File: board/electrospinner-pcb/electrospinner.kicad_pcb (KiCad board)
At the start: 2 copper layers, 50.8 x 38.1 mm, 35 parts, among them SW1 ResetBTN, U1 FT230XS, U2 TPS62147, U3 TPS62147, U4 A4988SETTR-T, U5 MSP430G2553IPW20

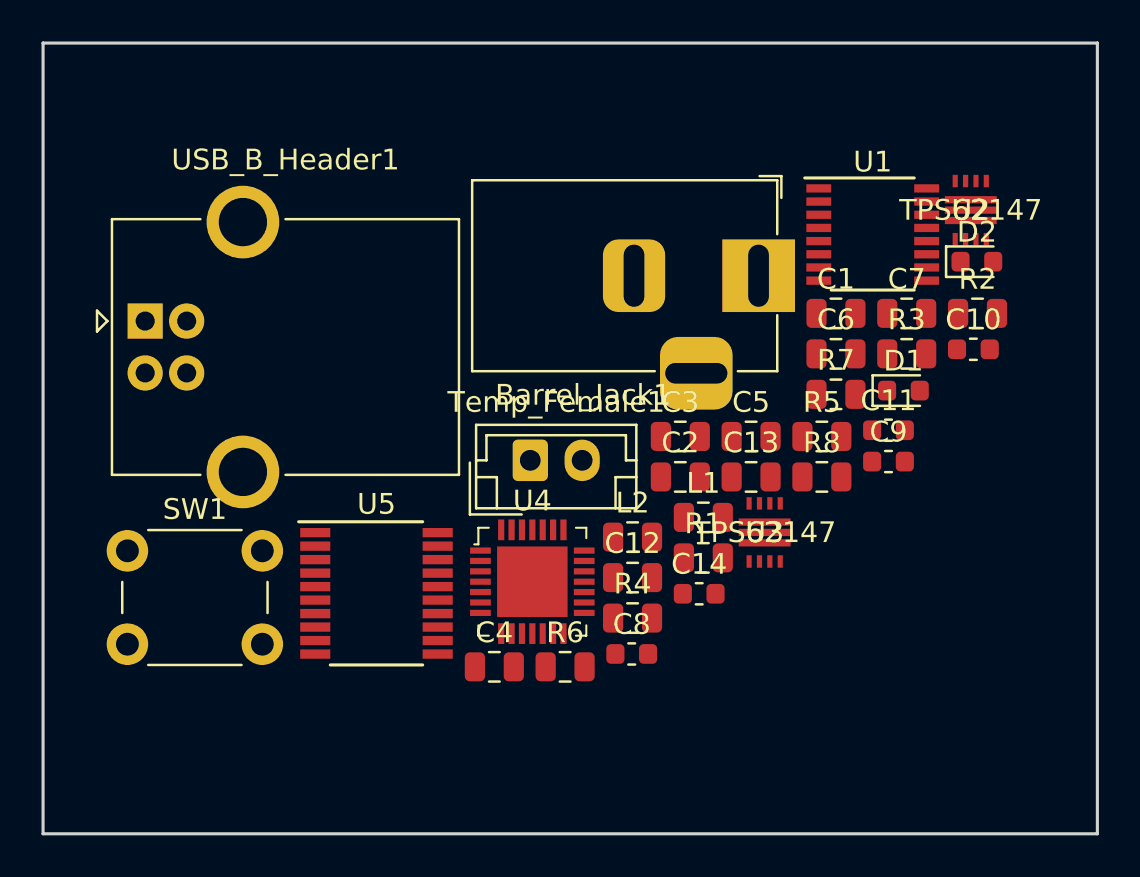
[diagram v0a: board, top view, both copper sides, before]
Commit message: Updates BOM and footprints, adds spreadsheet
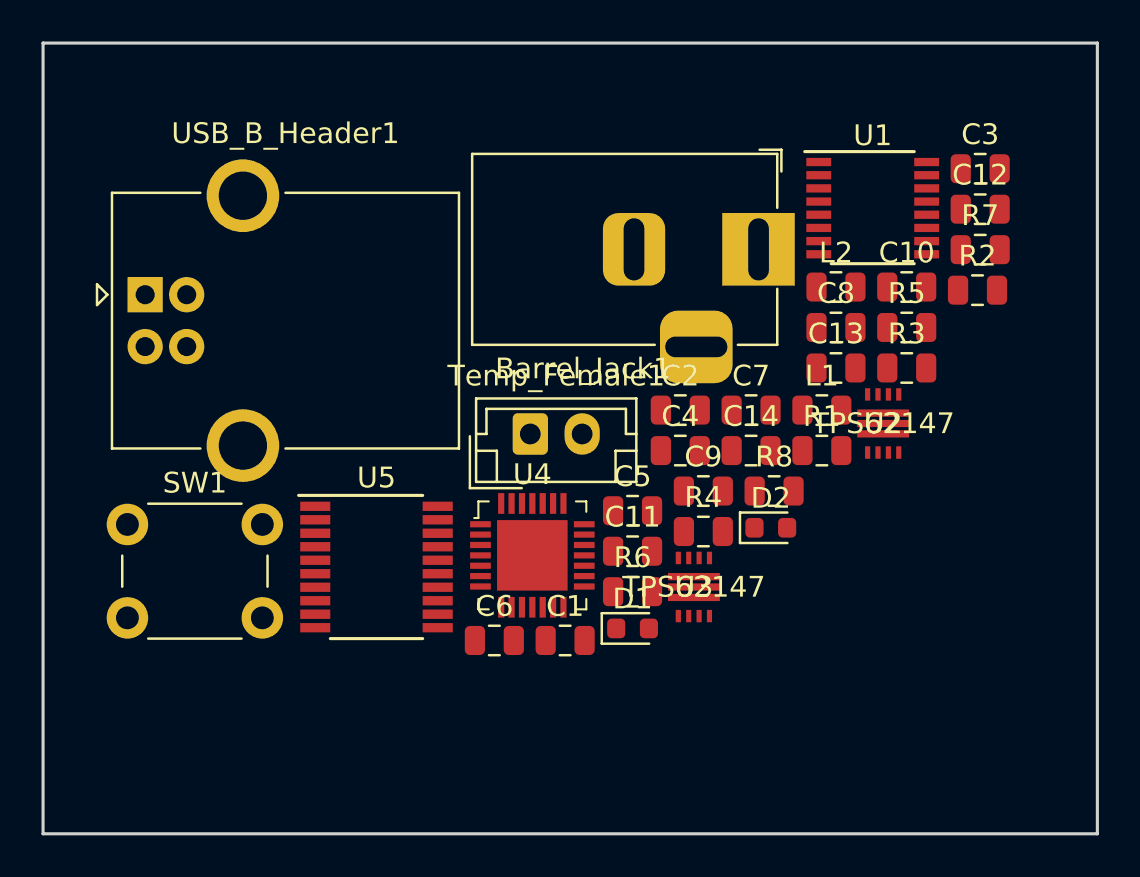
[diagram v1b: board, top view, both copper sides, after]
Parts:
- C10, C11, C14, C8, C9: footprint Capacitor_SMD:C_0603_1608Metric -> Capacitor_SMD:C_0805_2012Metric
- C5, C6: value 2uF -> 2.2uF
- moved C12 24.4 mm to (172.2, 96.9)
- moved C6 21.5 mm to (148.7, 117.7)
- moved C1 20.5 mm to (152.2, 117.7)
- moved C3 19.4 mm to (172.2, 95.0)
- moved C8 18.6 mm to (165.2, 102.6)
- moved D1 17.4 mm to (155.4, 117.1)
- moved D2 16.2 mm to (162.1, 112.3)
- moved L2 15.5 mm to (165.2, 100.7)
- moved C4 13.7 mm to (157.7, 108.5)
- moved C11 13.6 mm to (155.4, 113.4)
- moved U2 11.1 mm to (167.5, 107.2)
- moved R7 9.84 mm to (172.2, 98.9)
- moved C9 9.03 mm to (158.8, 110.5)
- moved C7 8.83 mm to (161.1, 106.6)
- moved R1 7.70 mm to (164.5, 108.5)
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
